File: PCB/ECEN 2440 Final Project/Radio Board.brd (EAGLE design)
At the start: 58.4 x 33 mm, 20 parts

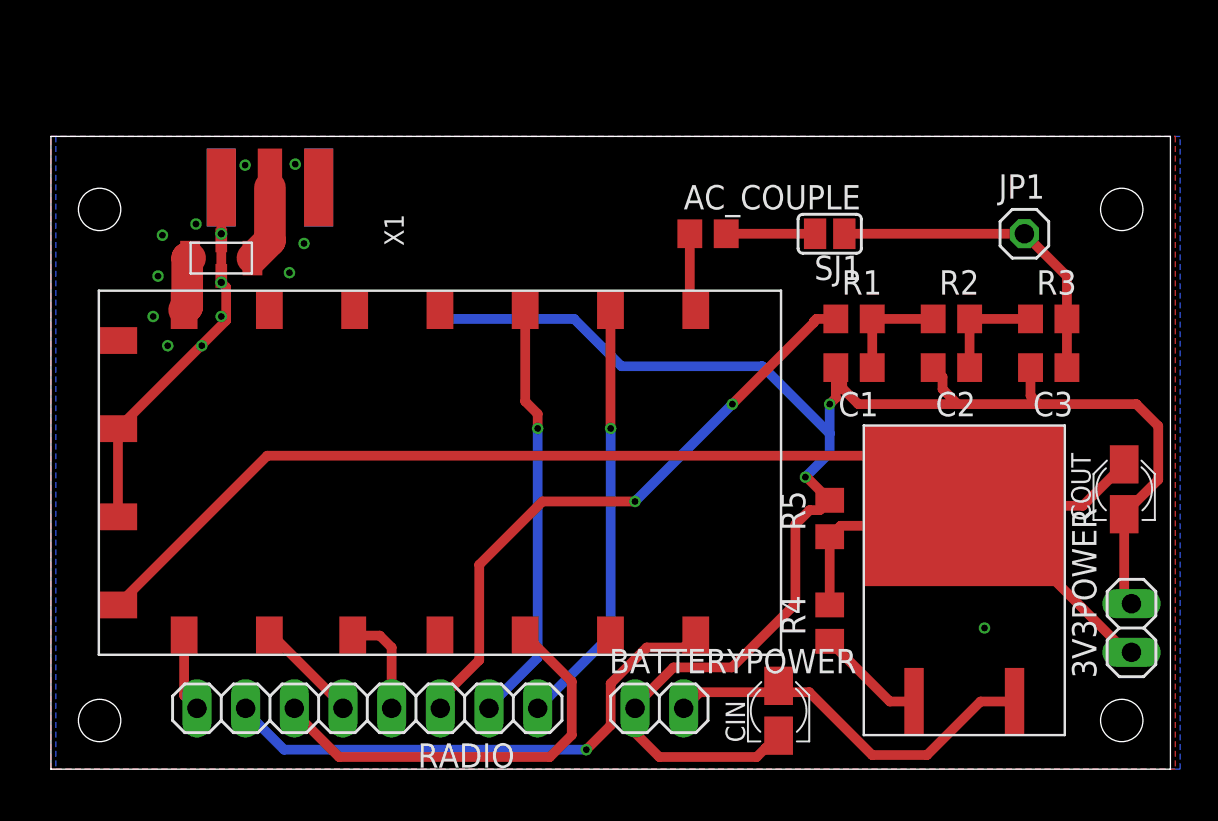
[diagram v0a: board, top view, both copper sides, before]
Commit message: final (before review & order) dra818v breakout board
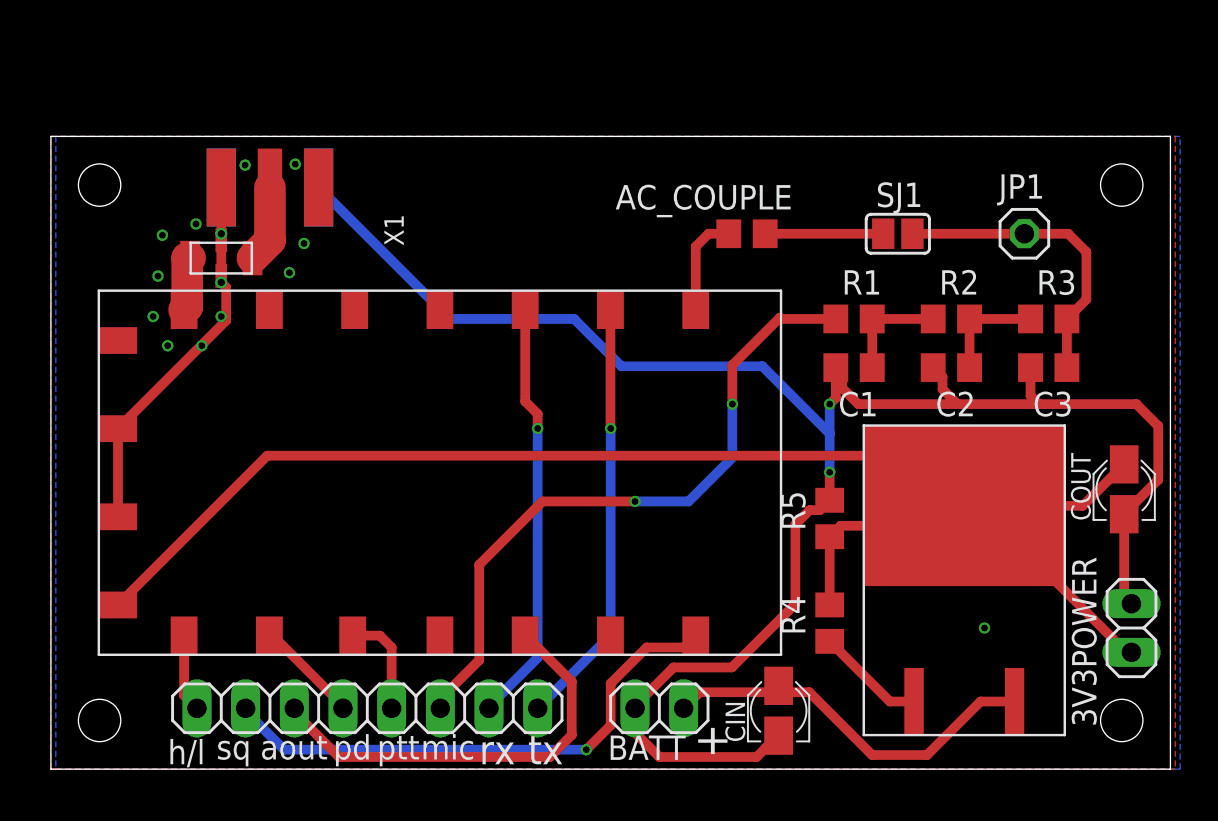
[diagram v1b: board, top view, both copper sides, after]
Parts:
- moved SJ1 3.56 mm to (44.2, 27.9)
- moved AC_COUPLE 2.03 mm to (36.3, 27.9)
- renumbered BATTERYPOWER to BATT
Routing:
- net GND: track 111.8 -> 119.5 mm
- net AUDIO_PWM: track 32.3 -> 35.2 mm
- net N$7: track 4.64 -> 6.16 mm
- net N$3: track 17.3 -> 15.9 mm
- net N$5: track 4.10 -> 5.30 mm
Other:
- board text added: "+"
- board text added: "aout"
- board text added: "h/l"
- board text added: "mic"
- board text added: "pd"
- board text added: "ptt"
- board text added: "rx"
- board text added: "sq"
- board text added: "tx"

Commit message: final (i hope) radio board
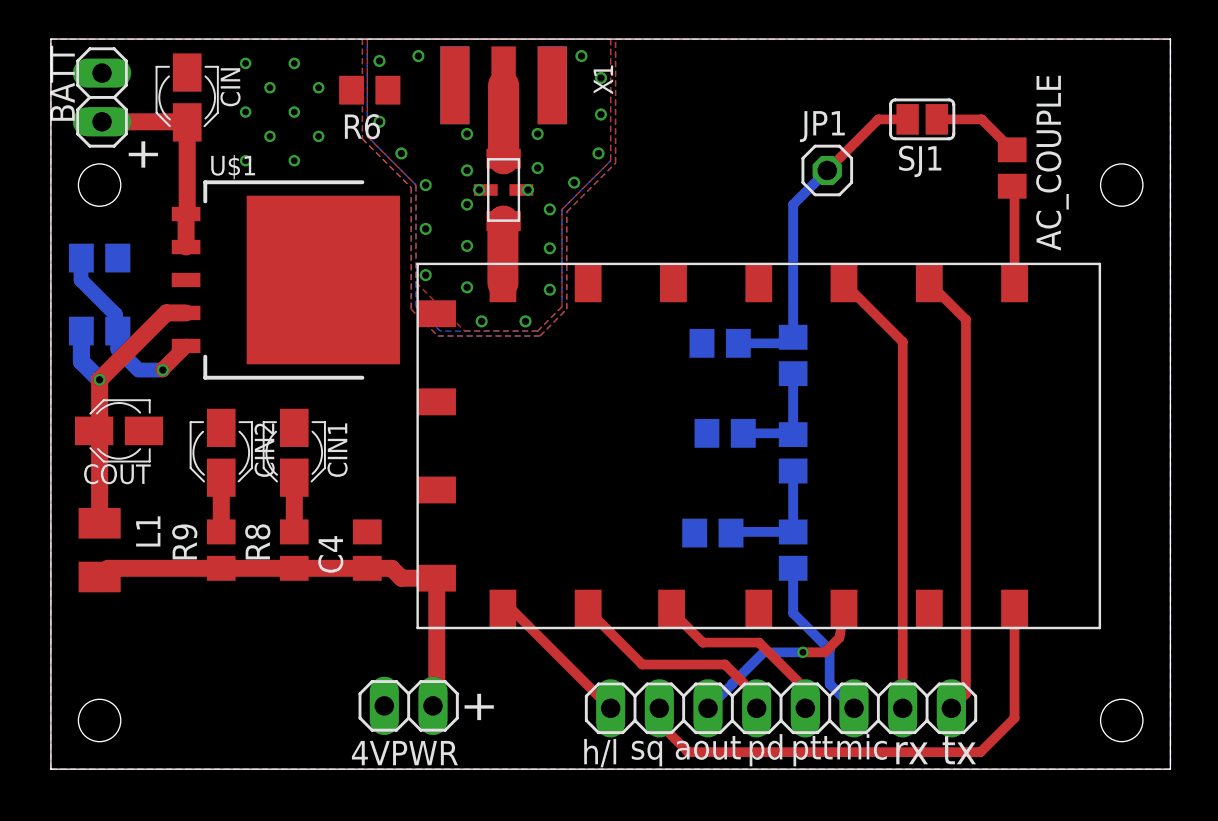
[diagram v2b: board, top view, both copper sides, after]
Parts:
- removed 3V3POWER: (no value), pinhead:1X02
- removed LM317: LM317, Custom Library:LM317
- added 4VPWR: (no value), pinhead:1X02
- added C4: 500n, rcl:C0805
- added CIN1, CIN2: (no value), rcl:PANASONIC_A
- added L1: (no value), rcl:L3225M
- added R6: 0R, rcl:R0805
- added R8, R9: (no value), rcl:R0805
- added U$1: BD00COAW, Custom Library:HRP5
- R4: value 220R -> 43k
- R5: value 470R -> 10k
- moved COUT 52.5 mm to (3.56, 17.7), turned to 180 degrees
- moved CIN 44.5 mm to (7.11, 35.1), turned to 270 degrees
- moved BATT 43.2 mm to (2.67, 35.1), turned to 270 degrees
- moved R4 41.0 mm to (2.54, 22.9), flipped to the bottom, turned to 180 degrees
- moved R5 40.5 mm to (2.54, 26.7), flipped to the bottom, turned to 180 degrees
- moved RADIO 21.6 mm to (38.1, 3.17)
- moved C3 17.2 mm to (34.9, 22.2), flipped to the bottom, turned to 0 degrees
- moved U$4 16.7 mm to (54.7, 7.37)
- moved U$6 15.2 mm to (23.6, 30.2), turned to 90 degrees
- moved AC_COUPLE 14.3 mm to (50.2, 31.4), turned to 90 degrees
- moved R3 13.5 mm to (38.7, 21.6), flipped to the bottom, turned to 90 degrees
- moved X1 13.3 mm to (23.6, 37.7)
- moved R1 12.5 mm to (38.7, 11.4), flipped to the bottom, turned to 90 degrees
- moved C2 12.3 mm to (35.2, 17.5), flipped to the bottom, turned to 0 degrees
- moved C1 11.4 mm to (34.5, 12.3), flipped to the bottom, turned to 0 degrees
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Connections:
- removed net +3V3: 3V3POWER.1, COUT.+, LM317.VOUT, R4.2, R5.1, U$4.VBAT
- new net ADJ: R4.2, R5.1, U$1.5
- new net GNDA: R6.1, U$6.GND1, U$6.GND2, U$6.P$1, U$6.P$2, X1.GND@1, X1.GND@2, X1.GND@3, X1.GND@4
- new net N$9: CIN1.+, R8.2
- new net V+: 4VPWR.1, C4.1, L1.2, R8.1, R9.1, U$4.VBAT
- new net VO: COUT.+, L1.1, R4.1, U$1.4
- net GND: now also 4VPWR.2, C4.2, CIN1.-, CIN2.-, R6.2, U$1.3, U$1.6; no longer 3V3POWER.2, U$6.GND1, U$6.GND2, U$6.P$1, U$6.P$2, X1.GND@1, X1.GND@2, X1.GND@3, X1.GND@4
- net N$8: now also CIN2.+, R9.2; no longer LM317.ADJUST1, R4.1
- net VCC: now also U$1.1, U$1.2; no longer LM317.VIN
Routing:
- net GND: track 119.5 -> 0.00 mm, vias 14 -> 10
- net +3V3: track 80.5 -> 0.00 mm
- net AUDIO_PWM: track 35.2 -> 8.62 mm, vias 2 -> 0
- net V+: track 0.00 -> 24.7 mm
- net VO: track 0.00 -> 16.6 mm, vias 0 -> 1
- net AF_OUT: track 22.3 -> 9.92 mm, vias 0 -> 1
- net ADJ: track 0.00 -> 10.1 mm, vias 0 -> 1
- net VCC: track 20.6 -> 11.0 mm
- net PD: track 5.49 -> 11.4 mm
- net AUDIO_PTT: track 5.46 -> 9.80 mm
- net H/L: track 4.07 -> 7.77 mm
- net N$8: track 5.70 -> 2.83 mm
- net N$9: track 0.00 -> 2.83 mm
- net SQ: track 28.2 -> 26.4 mm, vias 1 -> 0
- net N$3: track 15.9 -> 17.7 mm
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- added copper zone on layer 1, net GNDA
- added copper zone on layer 16, net GNDA
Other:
- board size 58.4 x 33 mm -> 58.4 x 38.1 mm
